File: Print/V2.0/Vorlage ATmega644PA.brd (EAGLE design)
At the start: 84 x 45 mm, 59 parts, among them IC1 ATmega644PA, IC4 ATTINY24/44/84-SSU, Q1 16MHz, X2 87758-0616

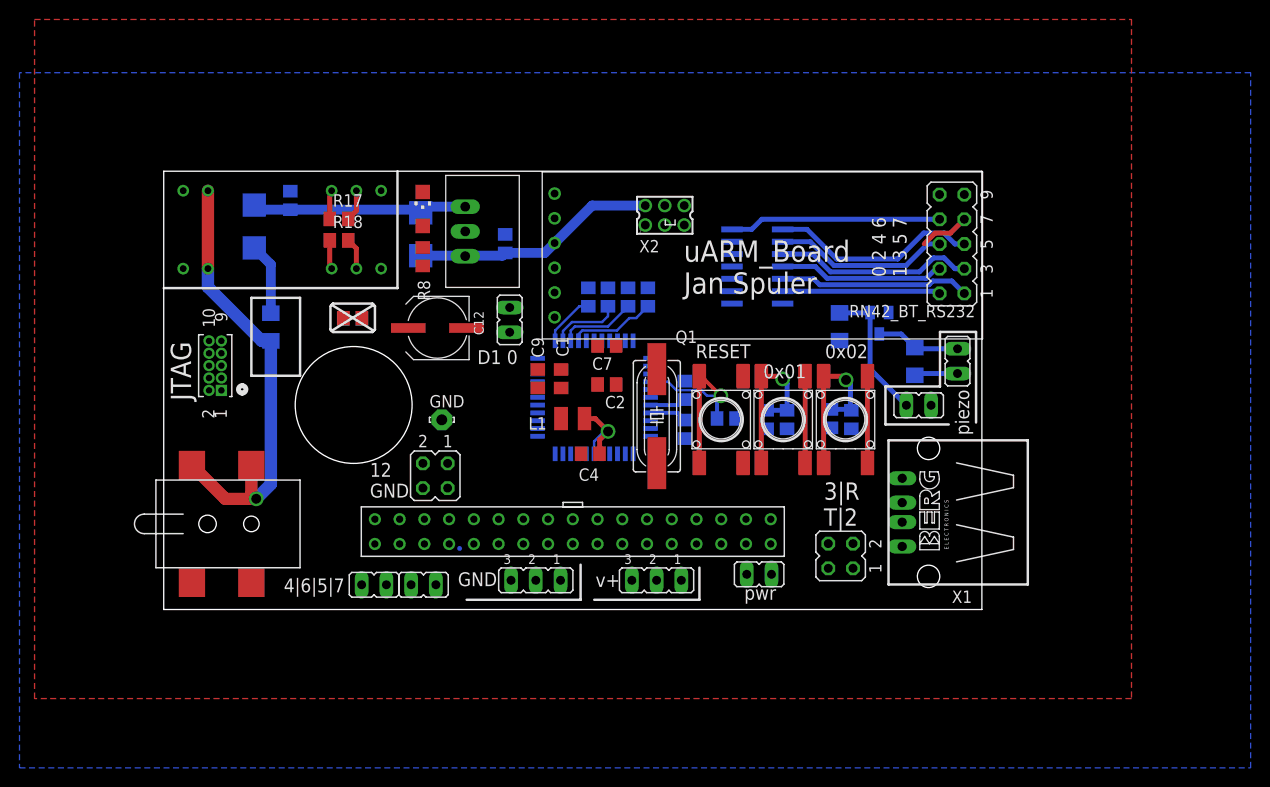
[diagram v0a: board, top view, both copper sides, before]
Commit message: print fertig
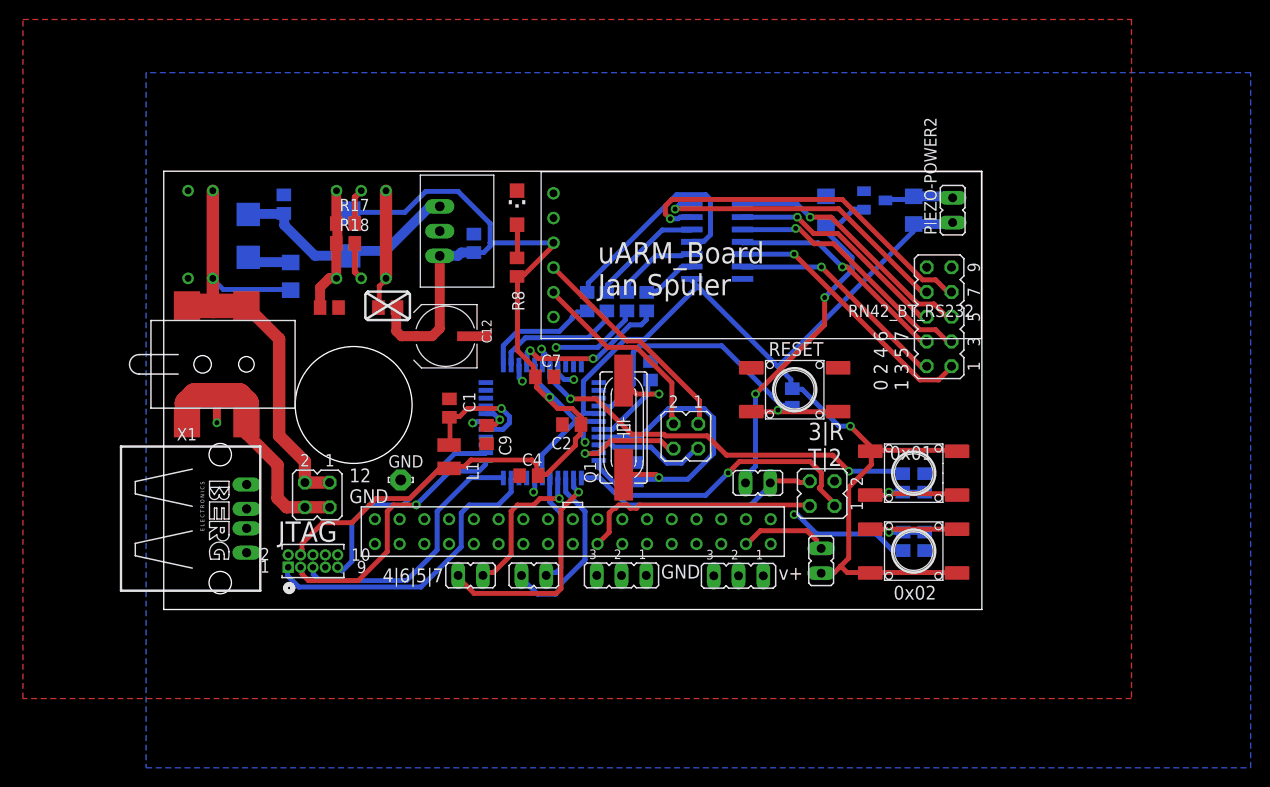
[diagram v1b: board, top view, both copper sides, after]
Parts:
- removed PIEZO-POWER6: (no value), jumper:JP1
- removed X2: 87758-0616, con-molex:87758-0616
- added JP2: (no value), jumper:JP2Q
- moved X1 72.7 mm to (5.80, 9.33), turned to 270 degrees
- moved JTAG 25.6 mm to (17.9, 5.61), turned to 0 degrees
- moved PIEZO-POWER1 18.3 mm to (61.0, 13.0)
- moved U$1 16.4 mm to (13.5, 25.2)
- moved R3 15.6 mm to (78.1, 13.0), turned to 270 degrees
- moved R21 15.5 mm to (77.0, 41.0)
- moved PIEZO-POWER2 15.5 mm to (81.0, 41.0)
- moved R1 15.4 mm to (75.9, 13.0), turned to 270 degrees
- moved S2 15.2 mm to (77.0, 6.00), turned to 0 degrees
- moved R2 14.6 mm to (75.9, 7.00)
- moved R4 14.6 mm to (78.1, 7.00)
- moved S1 14.5 mm to (77.0, 14.0), turned to 180 degrees
- moved L1 13.3 mm to (29.3, 15.7), turned to 90 degrees
- moved V12 12.6 mm to (73.0, 42.0), turned to 90 degrees
- moved JP3 12.3 mm to (15.8, 11.8)
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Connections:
- net PB0_ renamed N$7
- net PB1_ renamed N$6
- net PB2_ renamed N$5
- removed net PB3_: IC4.4, R10.2, X2.5
- new net N$14: JP2.3, RN1.5
- new net N$15: JP2.1, RN1.4
- new net N$3: IC4.4, R10.2
- net GND: no longer X2.6
- net PA4_: no longer X2.3
- net PA5_: no longer X2.1
- net PA6_: no longer X2.4
- net PD0: now also JP2.2; no longer PIEZO-POWER6.2, RN1.4
- net PD1: now also JP2.4; no longer PIEZO-POWER6.1, RN1.5
- net VCC: no longer X2.2
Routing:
- net VCC: track 56.3 -> 233.4 mm, vias 1 -> 2
- net RX: track 0.00 -> 62.0 mm
- net TX: track 0.00 -> 59.8 mm
- net DGND: track 5.96 -> 51.3 mm, vias 0 -> 5
- net PB1: track 0.00 -> 43.9 mm, vias 0 -> 2
- net PB0: track 0.00 -> 41.7 mm, vias 0 -> 2
- net PA7_: track 5.15 -> 37.4 mm, vias 0 -> 1
- net PC2: track 0.00 -> 31.9 mm
- net PD2: track 0.00 -> 30.9 mm, vias 0 -> 1
- net PC4: track 0.00 -> 27.7 mm, vias 0 -> 1
- net PC3: track 0.00 -> 27.2 mm
- net N$36: track 3.82 -> 30.1 mm, vias 0 -> 1
- net PD3: track 0.00 -> 26.0 mm
- net PD4: track 0.00 -> 24.0 mm, vias 0 -> 1
- net N$3: track 0.00 -> 23.3 mm
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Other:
- board text removed: "D1 0"
- board text removed: "piezo"
- board text removed: "pwr"
